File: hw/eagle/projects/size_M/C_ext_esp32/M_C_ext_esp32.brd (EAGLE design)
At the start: 19 parts, among them IC1 CP2102

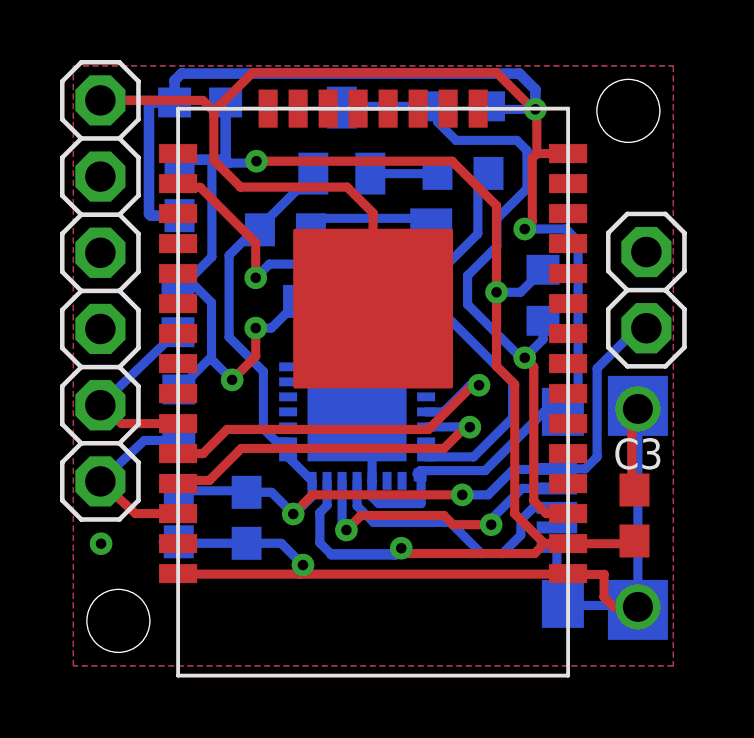
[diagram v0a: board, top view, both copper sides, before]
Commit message: pcb M.1 -not finished
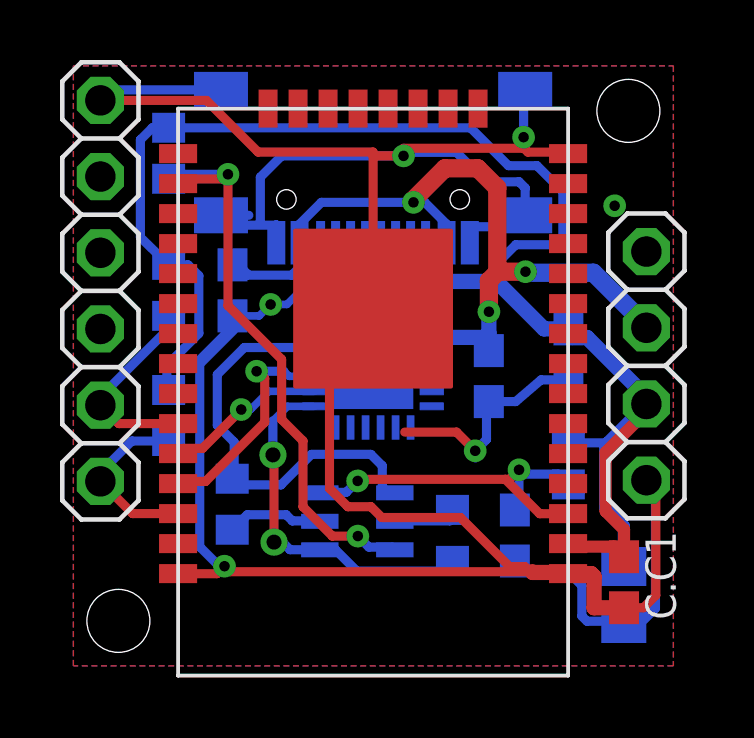
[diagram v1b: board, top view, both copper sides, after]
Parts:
- removed C1, C2, C4: 100n, rcl:C0603
- removed C3: 0.1F, rcl:C0603
- removed C5: 10u, rcl:C0603
- removed C6: 2u2, rcl:C0603
- removed IC1: CP2102, silabs:MLP28
- removed R1, R2: 2k2, rcl:R0603
- removed R3, R4, R5, R6: 12k, rcl:R0603
- removed T1, T2: (no value), transistor:SOT23-BEC
- removed USB: MICRO-USB, hugo:MICRO-USB
- added C.C1, C.C2, C.C4: 100n, rcl:C0603
- added C.C3: 22u, rcl:C0805
- added C.C5: 10u, rcl:C0603
- added C.C6: 2u2, rcl:C0603
- added C.R1, C.R2: 2k2, rcl:R0603
- added C.R3, C.R4, C.R5, C.R6: 12k, rcl:R0603
- added C.U1: TTGO-MICRO-32, hugo:TTGO-MICRO-32
- added C.U3: BC817DS,115, SamacSys_Parts:SOT95P275X110-6N
- added U1: CP2104-F03-GM, CP2104:QFN50P400X400X80-25N
- JP1: device pinhead2:1X02 -> pinhead2:1X04
- U$1: value TTGO-MICRO-32 -> USB-C; device hugo:TTGO-MICRO-32 -> hugo:USB-C
- moved U$1 8.85 mm to (10.5, 18.4), flipped to the bottom
- moved JP1 2.53 mm to (19.6, 10.5)
- renumbered JP2 to C.J2
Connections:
- removed net VDD: C1.1, C2.1, C3.1, IC1.6, R1.2, R2.2, R5.2, R6.1, U$1.3V3
- new net VCC: C.C1.1, C.C2.1, C.C3.1, C.R1.2, C.R2.2, C.R5.2, C.R6.1, C.U1.3V3, JP1.3, U1.6
- new net VIO: U1.5
- net GND: now also C.C1.2, C.C2.2, C.C3.2, C.C4.1, C.C5.1, C.C6.2, C.U1.GND1, C.U1.GND10, C.U1.GND11, C.U1.GND2, C.U1.GND3, C.U1.GND4, C.U1.GND5, C.U1.GND6, C.U1.GND7, C.U1.GND8, C.U1.GND9, JP1.4, U$1.A1B12, U$1.B1A12, U$1.SH1, U$1.SH2, U$1.SH3, U$1.SH4, U1.2, U1.25; no longer C1.2, C2.2, C3.2, C4.1, C5.1, C6.2, IC1.3, IC1.EXP, IC1.M, U$1.GND1, U$1.GND2, U$1.GND3, U$1.GND4, USB.GND, USB.GND1, USB.GND2, USB.GND3, USB.GND4, USB.P$1, USB.P$2
- net N$1: now also U$1.A7, U1.4; no longer IC1.5, USB.D-
- net N$10: now also C.R5.1, C.U1.IO0, C.U3.3; no longer R5.1, T2.C, U$1.IO0
- net N$11: now also C.C6.1, C.R6.2, C.U1.EN, C.U3.6; no longer C6.1, R6.2, T1.C, U$1.EN
- net N$13: now also C.U1.IO2; no longer U$1.IO2
- net N$2: now also U$1.A6, U1.3; no longer IC1.4, USB.D+
- net N$5: now also C.R4.2, C.U3.5; no longer R4.2, T1.B
- net N$7: now also C.R3.2, C.U3.2; no longer R3.2, T2.B
- net N$8: now also C.R3.1, C.U3.4, U1.19; no longer IC1.9, R3.1, T1.E
- net N$9: now also C.R4.1, C.U3.1, U1.23; no longer IC1.28, R4.1, T2.E
- net RX: now also C.U1.RXD0, U1.20; no longer IC1.25, U$1.RXD0
- net SCL: now also C.R1.1, C.U1.IO22; no longer R1.1, U$1.IO22
- net SDA: now also C.R2.1, C.U1.IO21; no longer R2.1, U$1.IO21
- net TX: now also C.U1.TXD0, U1.21; no longer IC1.26, U$1.TXD0
- net VUSB: now also C.C4.2, C.C5.2, U$1.A4B9, U$1.B4A9, U1.7, U1.8; no longer C4.2, C5.2, IC1.7, IC1.8, USB.VUSB
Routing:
- net VCC: track 0.00 -> 56.4 mm
- net VDD: track 54.9 -> 0.00 mm, vias 5 -> 0
- net N$11: track 23.4 -> 12.9 mm, vias 1 -> 2
- net N$10: track 9.96 -> 19.7 mm, vias 1 -> 2
- net GND: track 111.2 -> 119.3 mm, vias 4 -> 6
- net RX: track 13.1 -> 5.41 mm
- net N$1: track 9.82 -> 2.26 mm, vias 2 -> 0
- net VUSB: track 22.7 -> 29.8 mm, vias 2 -> 3
- net N$2: track 9.08 -> 2.25 mm
- net TX: track 12.0 -> 7.57 mm
- net N$7: track 4.91 -> 2.24 mm
- net N$9: track 13.5 -> 14.6 mm
- net N$8: track 11.2 -> 12.3 mm, vias 0 -> 2
- net N$5: track 2.51 -> 3.22 mm
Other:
- board text added: "ESP M.1"
- board text removed: "esp M.0"
